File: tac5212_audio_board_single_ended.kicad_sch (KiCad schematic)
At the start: 94 parts, among them J1002 TAC5212, U1 Single Buffer - 74LVC1G125GV,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, U2 3.3v LDO - TLV74133PDQNR

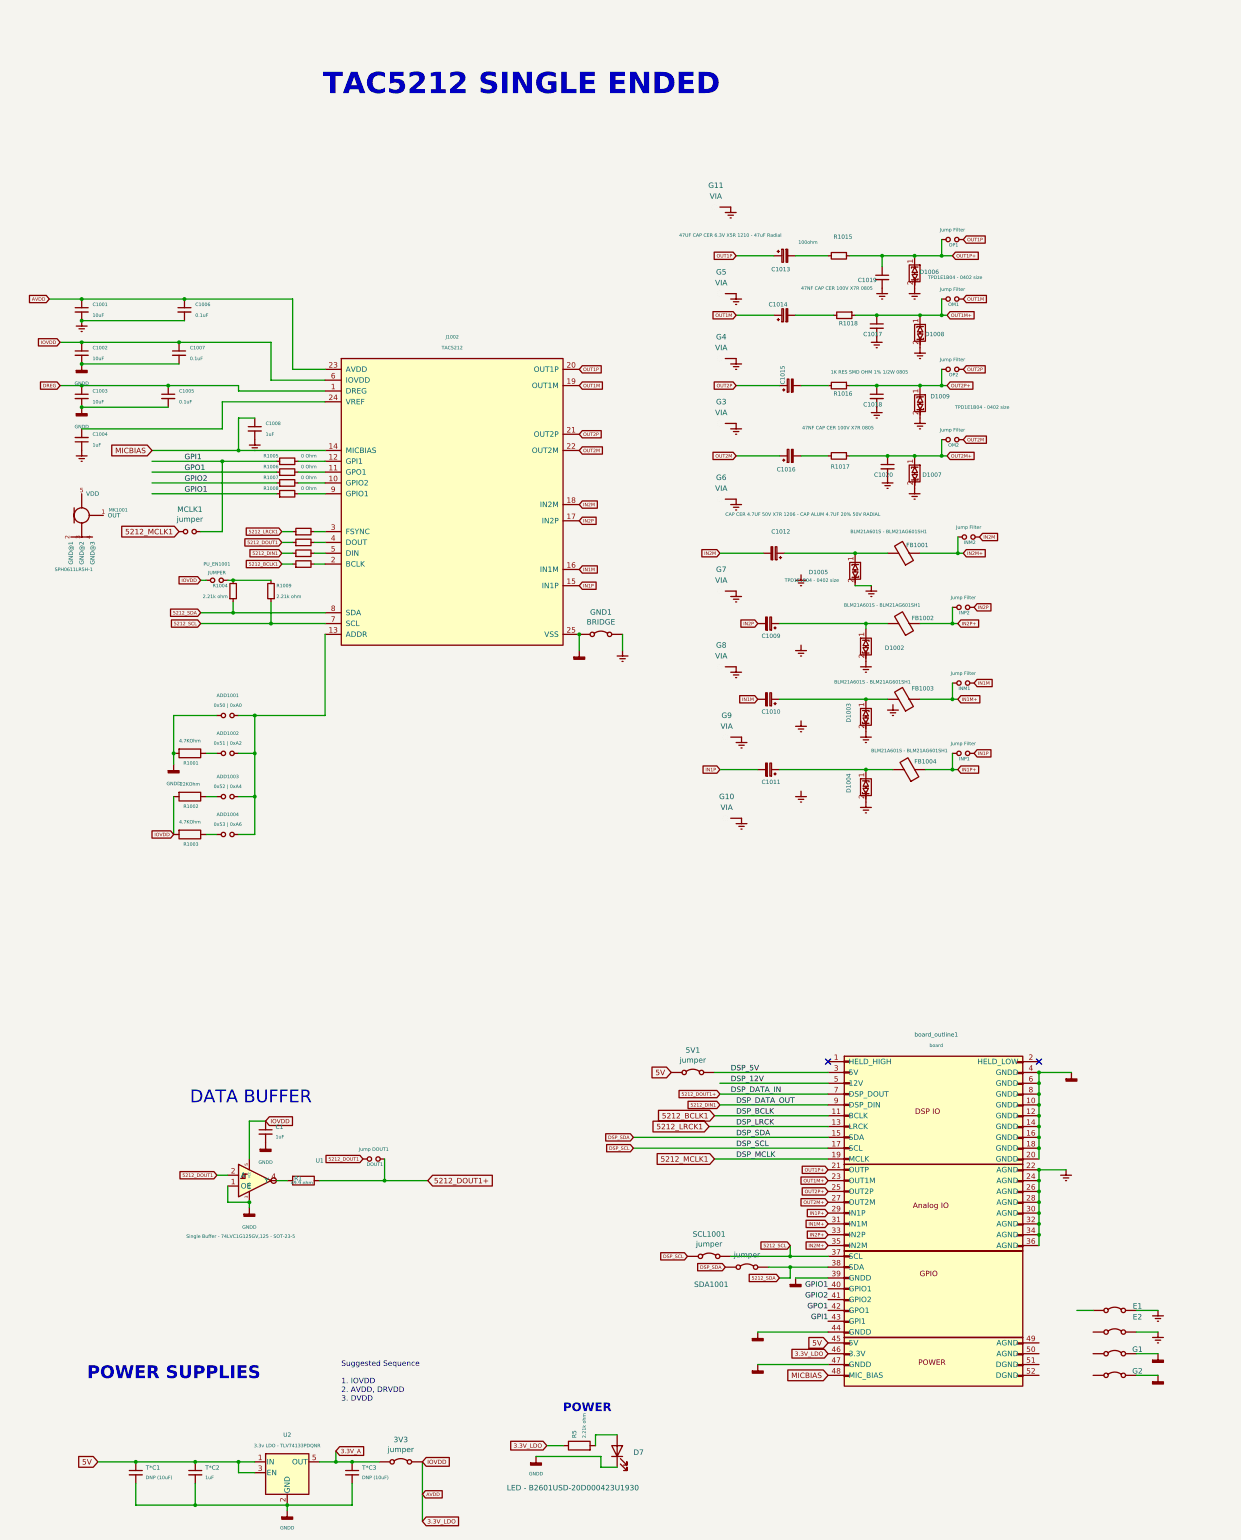
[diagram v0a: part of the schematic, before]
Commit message: update
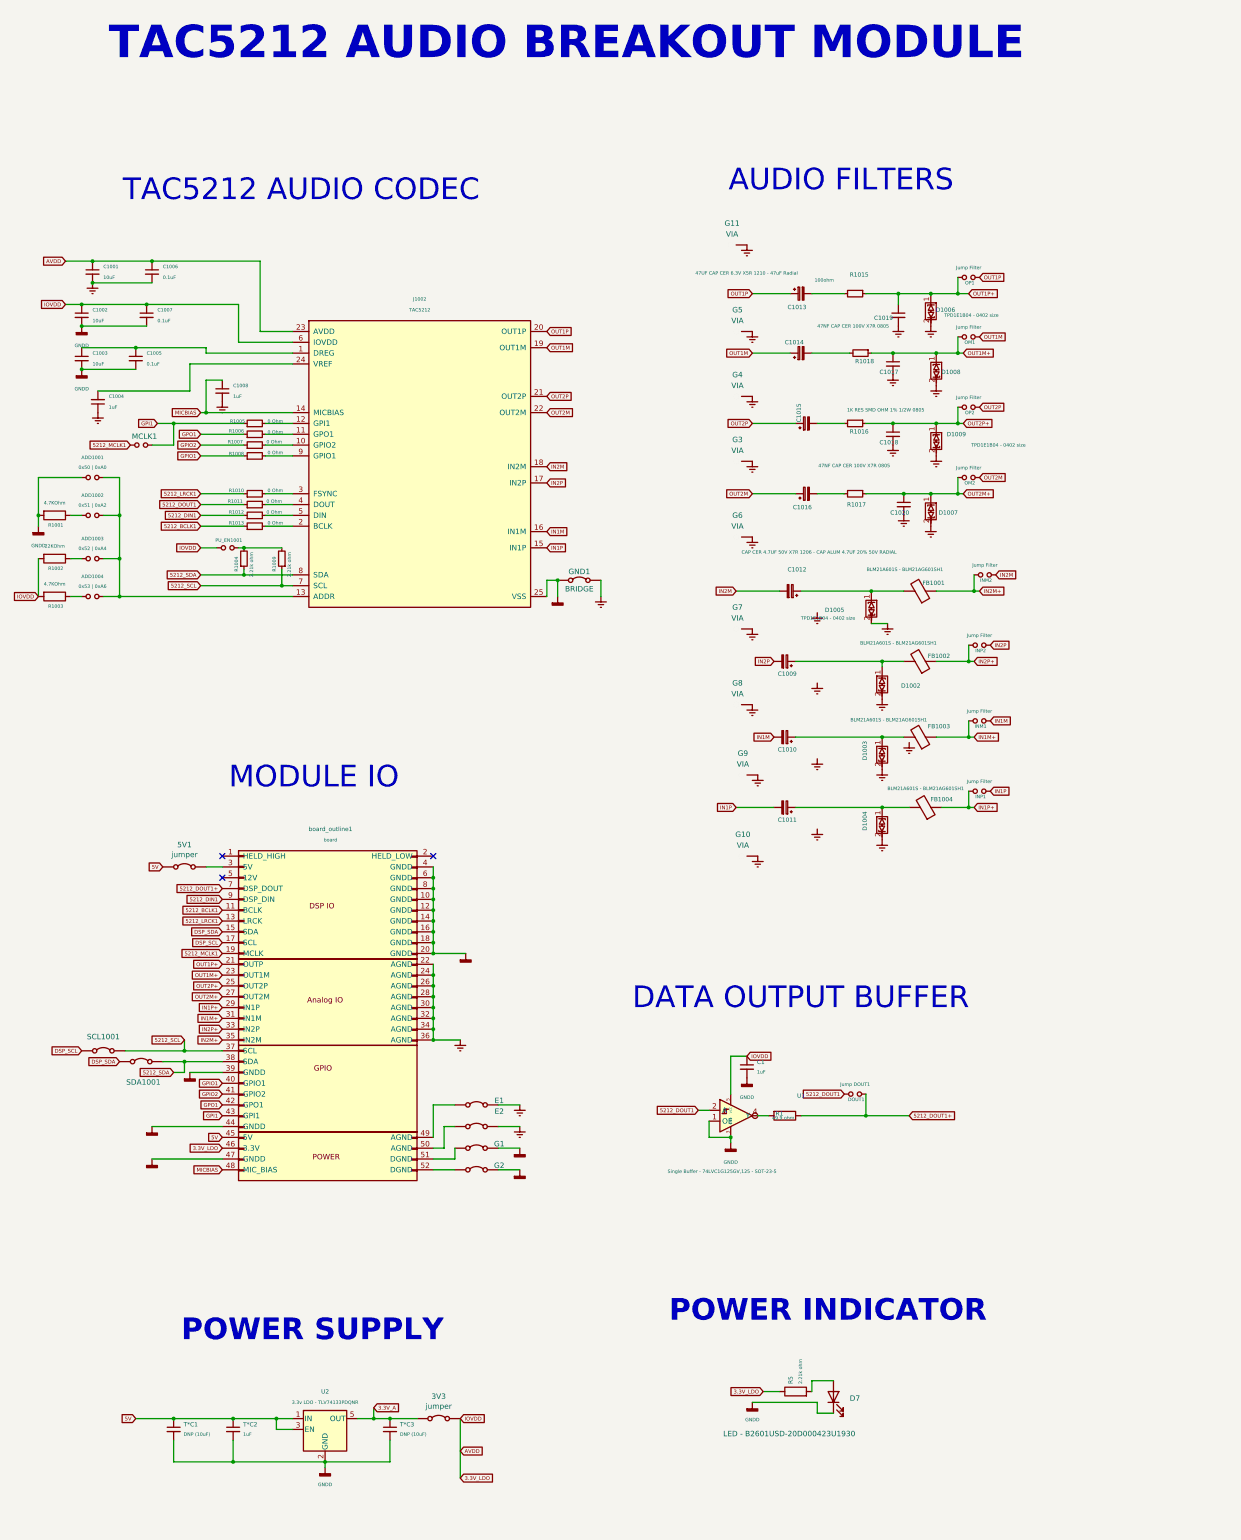
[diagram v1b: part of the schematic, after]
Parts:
- removed MK1001: SPH0611LR5H-1, SPH0611LR5H-1:XDCR_SPH0611LR5H-1, symbol proejct_lib:SPH0611LR5H-1
- 3V3, 5V1, E1, E2, G1, G2, GND1, MCLK1, SCL1001, SDA1001: PCBWAY_2020-06-09 NO COMPONENT -> (none); PCBWAY_2020-08-27 NO COMPONENT -> (none); PCBWAY_2020_04_18 NO COMPONENT -> (none)
- ADD1001, ADD1002, ADD1003, ADD1004, D1002, D1003, D1004, D1006, D1007, D1008, D1009, DOUT1, INM1, INM2, INP1, INP2, OM1, OM2, OP1, OP2, PU_EN1001: Part Number 2020-05-29 NO COMPONENT -> (none); Part Number 2020-08-26 NO COMPONENT -> (none); Part Number 2020-09-07 NO NEED TO PURCHASE OR MOUNT -> (none)
- C1: Manufacturer KEMET -> (none); Manufacturer_Part_Number C0805C104K5RAC7411 -> (none); mouser 80-C0805C104K5RACLR -> (none)
- C1010, C1011, C1013, C1014: 2024-01-06 UUQ1C100MCL1GB -> (none)
- C1012: SPEC CAP_100u_20%_25V_ALUM_RADIAL -> (none)
- C1015: Manufacturer Wurth Elektronik -> (none); Manufacturer_Part_Number 860020472006 -> (none); mouser 710-860020472006 -> (none)
- C1016, C1017, C1018, C1019, C1020: Digikey C1608X7R1H473K -> (none); Manufacturer TDK -> (none); Manufacturer_Part_Number C1608X7R1H473K080AA -> (none); mouser 810-C1608X7R1H473K -> (none)
- R1: mouser 603-RC0805DR-072K2L -> (none)
- R1001, R1002, R1003: Part Number 2020-05-29 ERJ-UP3J222V -> (none); Part Number 2020-08-26 ERJ-PA2F2211X (2.21k) -> (none); Part Number 2020-09-07 ERJ-PA2F2211X (2.21k) -> (none)
- R1016, R1018: Digikey ERJ-3EKF1000V -> (none); Manufacturer Bourns -> (none); Manufacturer_Part_Number CMP0805AFX-1000ELF -> (none); mouser 652-CMP0805AFX-1000L -> (none)
- R5: Digikey P100BYCT-ND -> (none); Manufacturer Bourns -> (none); Manufacturer_Part_Number CMP0805AFX-1000ELF -> (none); mouser 652-CMP0805AFX-1000L -> (none)
- T*C1, T*C3: Manufacturer Taiyo Yuden -> (none); Manufacturer_Part_Number LMR212BD7106KG-T -> (none); mouser 963-LMR212BD7106KG-T -> (none)
- T*C2: Manufacturer Kyocera AVX -> (none); Manufacturer_Part_Number 08055C104M4T4A -> (none); mouser 581-08055C104M4T4A -> (none)
- U1: Manufacturer TI / Nexperia -> (none); Manufacturer_Part_Number 74LVC1G125GV,125 -> (none); mouser 771-74LVC1G125GV -> (none)
- board_outline1: Digikey - -> (none); Manufacturer - -> (none); Manufacturer_Part_Number - -> (none); mouser - -> (none)
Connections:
- net at G1.1 (A): now also board_outline1.51 (DGND)
- net at board_outline1.49 (AGND): now also E1.1 (A)
- net at board_outline1.50 (AGND): now also E2.1 (A)
- net at board_outline1.52 (DGND): now also G2.1 (A)
- net DREG: no longer names the net of C1003.1, C1005.1, J1002.1 (DREG)
- net DSP_12V: no longer names the net of board_outline1.5 (12V)
- net DSP_5V: no longer names the net of 5V1.2 (B), board_outline1.3 (5V)
- no-connect marks 2 -> 3
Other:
- note added: "AUDIO FILTERS"
- note added: "DATA OUTPUT BUFFER"
- note added: "MODULE IO"
- note added: "POWER INDICATOR"
- note added: "POWER SUPPLY"
- note added: "TAC5212 AUDIO BREAKOUT MODULE"
- note added: "TAC5212 AUDIO CODEC"
- note removed: "DATA BUFFER"
- note removed: "POWER"
- note removed: "POWER SUPPLIES"
- note removed: "Suggested Sequence 1. IOVDD 2. AVDD, DRVDD 3. DVDD"
- note removed: "TAC5212 SINGLE ENDED"
- moved on the sheet: 3V3, 5V1, ADD1001, ADD1002, ADD1003, ADD1004, C1, C1001, C1002, C1003, C1004, C1005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
